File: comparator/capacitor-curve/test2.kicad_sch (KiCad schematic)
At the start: 4 parts

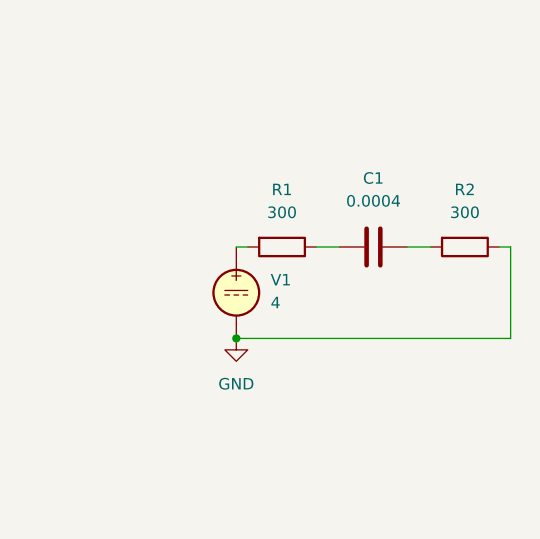
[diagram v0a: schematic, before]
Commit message: add/fix
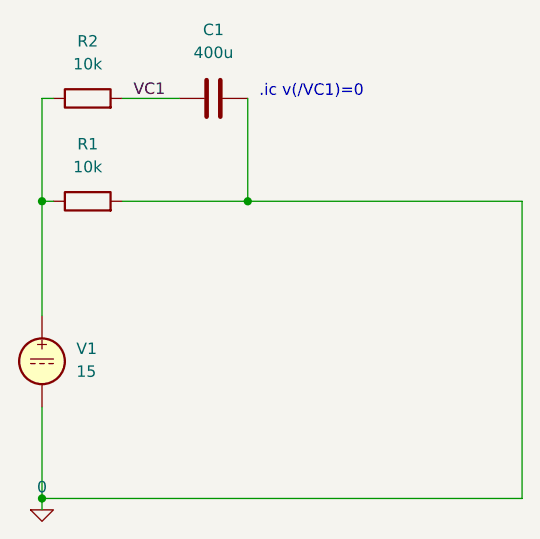
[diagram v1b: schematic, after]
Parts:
- C1: value 0.0004 -> 400u
- R1, R2: value 300 -> 10k
- V1: value 4 -> 15
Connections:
- net at R1.1: now also R2.1, V1.1; no longer C1.1
- net 0: now reaches C1.2
- net 0: now also R1.2, V1.2; no longer R2.2
- removed net GND: R2.1, V1.2
- new net VC1: C1.1, R2.2
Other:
- note added: ".ic v(/VC1)=0"
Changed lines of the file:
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@@
 (kicad_sch (version 20230121) (generator eeschema)
   (paper "A4")
-  (junction (at 81.28 90.17) (diameter 0) (color 0 0 0 0)
+  (junction (at 59.69 74.93) (diameter 0) (color 0 0 0 0)
   )
-  (wire (pts (xy 81.28 80.01) (xy 82.55 80.01))
+  (junction (at 82.55 74.93) (diameter 0) (color 0 0 0 0)
+  )
+  (junction (at 59.69 107.95) (diameter 0) (color 0 0 0 0)
+  )
+  (wire (pts (xy 113.03 107.95) (xy 113.03 74.93))
     (stroke (width 0) (type default))
   )
-  (wire (pts (xy 92.71 80.01) (xy 90.17 80.01))
+  (wire (pts (xy 59.69 109.22) (xy 59.69 107.95))
     (stroke (width 0) (type default))
   )
-  (wire (pts (xy 111.76 80.01) (xy 111.76 90.17))
+  (wire (pts (xy 59.69 87.63) (xy 59.69 74.93))
     (stroke (width 0) (type default))
   )
-  (wire (pts (xy 110.49 80.01) (xy 111.76 80.01))
+  (wire (pts (xy 59.69 97.79) (xy 59.69 107.95))
     (stroke (width 0) (type default))
   )
-  (wire (pts (xy 100.33 80.01) (xy 102.87 80.01))
+  (wire (pts (xy 59.69 74.93) (xy 60.96 74.93))
     (stroke (width 0) (type default))
   )
-  (wire (pts (xy 111.76 90.17) (xy 81.28 90.17))
+  (wire (pts (xy 59.69 63.5) (xy 60.96 63.5))
     (stroke (width 0) (type default))
   )
-  (symbol (lib_id "Device:C") (at 96.52 80.01 90) (unit 1)
+  (wire (pts (xy 82.55 74.93) (xy 113.03 74.93))
+    (stroke (width 0) (type default))
+  )
+  (wire (pts (xy 82.55 63.5) (xy 82.55 74.93))
+    (stroke (width 0) (type default))
+  )
+  (wire (pts (xy 59.69 74.93) (xy 59.69 63.5))
+    (stroke (width 0) (type default))
+  )
+  (wire (pts (xy 68.58 74.93) (xy 82.55 74.93))
+    (stroke (width 0) (type default))
+  )
+  (wire (pts (xy 59.69 107.95) (xy 113.03 107.95))
+    (stroke (width 0) (type default))
+  )
+  (wire (pts (xy 68.58 63.5) (xy 74.93 63.5))
+    (stroke (width 0) (type default))
+  )
+  (text ".ic v(/VC1)=0" (at 83.82 63.5 0)
+    (effects (font (size 1.27 1.27)) (justify left bottom))
+  )
+  (label "VC1" (at 69.85 63.5 0) (fields_autoplaced)
+    (effects (font (size 1.27 1.27)) (justify left bottom))
+  )
+  (symbol (lib_id "Simulation_SPICE:VDC") (at 59.69 92.71 0) (unit 1)
     (in_bom yes) (on_board yes) (dnp no) (fields_autoplaced)
-    (property "Reference" "C1" (at 96.52 72.39 90)
+    (property "Reference" "V1" (at 63.5 91.3102 0)
+      (effects (font (size 1.27 1.27)) (justify left))
+    )
+    (property "Value" "15" (at 63.5 93.8502 0)
+      (effects (font (size 1.27 1.27)) (justify left))
+    )
+    (property "Footprint" "" (at 59.69 92.71 0)
+      (effects (font (size 1.27 1.27)) hide)
+    )
+    (property "Datasheet" "~" (at 59.69 92.71 0)
+      (effects (font (size 1.27 1.27)) hide)
+    )
+    (property "Sim.Pins" "1=+ 2=-" (at 59.69 92.71 0)
+      (effects (font (size 1.27 1.27)) hide)
+    )
+    (property "Sim.Type" "DC" (at 59.69 92.71 0)
+      (effects (font (size 1.27 1.27)) hide)
+    )
+    (property "Sim.Device" "V" (at 59.69 92.71 0)
+      (effects (font (size 1.27 1.27)) (justify left) hide)
+    )
+    (pin "1")
+    (pin "2")
+    (instances
+      (project "test2"
+        (path "/bb173b4d-9621-4ad4-b8d6-5552f010e489"
+          (reference "V1") (unit 1)
+        )
+      )
+    )
+  )
+  (symbol (lib_id "Device:C") (at 78.74 63.5 90) (unit 1)
+    (in_bom yes) (on_board yes) (dnp no) (fields_autoplaced)
+    (property "Reference" "C1" (at 78.74 55.88 90)
       (effects (font (size 1.27 1.27)))
     )
-    (property "Value" "0.0004" (at 96.52 74.93 90)
+    (property "Value" "400u" (at 78.74 58.42 90)
       (effects (font (size 1.27 1.27)))
     )
-    (property "Footprint" "" (at 100.33 79.0448 0)
+    (property "Footprint" "" (at 82.55 62.5348 0)
       (effects (font (size 1.27 1.27)) hide)
     )
-    (property "Datasheet" "~" (at 96.52 80.01 0)
+    (property "Datasheet" "~" (at 78.74 63.5 0)
       (effects (font (size 1.27 1.27)) hide)
     )
@@
     (pin "2")
     (instances
-      (project "test-details"
-        (path "/8300bb89-af22-40bb-96f5-ff500b49d277"
+      (project "test2"
+        (path "/bb173b4d-9621-4ad4-b8d6-5552f010e489"
           (reference "C1") (unit 1)
         )
@@
     )
   )
-  (symbol (lib_id "Device:R") (at 106.68 80.01 270) (unit 1)
+  (symbol (lib_id "Device:R") (at 64.77 63.5 90) (unit 1)
     (in_bom yes) (on_board yes) (dnp no) (fields_autoplaced)
-    (property "Reference" "R2" (at 106.68 73.66 90)
+    (property "Reference" "R2" (at 64.77 57.15 90)
       (effects (font (size 1.27 1.27)))
     )
-    (property "Value" "300" (at 106.68 76.2 90)
+    (property "Value" "10k" (at 64.77 59.69 90)
       (effects (font (size 1.27 1.27)))
     )
-    (property "Footprint" "" (at 106.68 78.232 90)
+    (property "Footprint" "" (at 64.77 65.278 90)
       (effects (font (size 1.27 1.27)) hide)
     )
-    (property "Datasheet" "~" (at 106.68 80.01 0)
+    (property "Datasheet" "~" (at 64.77 63.5 0)
       (effects (font (size 1.27 1.27)) hide)
     )
@@
     (pin "2")
     (instances
-      (project "test-details"
-        (path "/8300bb89-af22-40bb-96f5-ff500b49d277"
+      (project "test2"
+        (path "/bb173b4d-9621-4ad4-b8d6-5552f010e489"
           (reference "R2") (unit 1)
         )
@@
     )
   )
-  (symbol (lib_id "Simulation_SPICE:VDC") (at 81.28 85.09 0) (unit 1)
+  (symbol (lib_id "Simulation_SPICE:0") (at 59.69 109.22 0) (unit 1)
     (in_bom yes) (on_board yes) (dnp no) (fields_autoplaced)
-    (property "Reference" "V1" (at 85.09 83.6902 0)
-      (effects (font (size 1.27 1.27)) (justify left))
-    )
-    (property "Value" "4" (at 85.09 86.2302 0)
-      (effects (font (size 1.27 1.27)) (justify left))
-    )
-    (property "Footprint" "" (at 81.28 85.09 0)
+    (property "Reference" "#GND01" (at 59.69 111.76 0)
       (effects (font (size 1.27 1.27)) hide)
     )
-    (property "Datasheet" "~" (at 81.28 85.09 0)
+    (property "Value" "0" (at 59.69 106.68 0)
+      (effects (font (size 1.27 1.27)))
+    )
+    (property "Footprint" "" (at 59.69 109.22 0)
       (effects (font (size 1.27 1.27)) hide)
     )
-    (property "Sim.Pins" "1=+ 2=-" (at 81.28 85.09 0)
+    (property "Datasheet" "~" (at 59.69 109.22 0)
       (effects (font (size 1.27 1.27)) hide)
     )
-    (property "Sim.Type" "DC" (at 81.28 85.09 0)
-      (effects (font (size 1.27 1.27)) hide)
-    )
-    (property "Sim.Device" "V" (at 81.28 85.09 0)
-      (effects (font (size 1.27 1.27)) (justify left) hide)
-    )
     (pin "1")
-    (pin "2")
     (instances
-      (project "test-details"
-        (path "/8300bb89-af22-40bb-96f5-ff500b49d277"
-          (reference "V1") (unit 1)
+      (project "test2"
+        (path "/bb173b4d-9621-4ad4-b8d6-5552f010e489"
+          (reference "#GND01") (unit 1)
         )
       )
     )
   )
-  (symbol (lib_id "Device:R") (at 86.36 80.01 270) (unit 1)
+  (symbol (lib_id "Device:R") (at 64.77 74.93 90) (unit 1)
     (in_bom yes) (on_board yes) (dnp no) (fields_autoplaced)
-    (property "Reference" "R1" (at 86.36 73.66 90)
+    (property "Reference" "R1" (at 64.77 68.58 90)
       (effects (font (size 1.27 1.27)))
     )
-    (property "Value" "300" (at 86.36 76.2 90)
+    (property "Value" "10k" (at 64.77 71.12 90)
       (effects (font (size 1.27 1.27)))
     )
-    (property "Footprint" "" (at 86.36 78.232 90)
+    (property "Footprint" "" (at 64.77 76.708 90)
       (effects (font (size 1.27 1.27)) hide)
     )
-    (property "Datasheet" "~" (at 86.36 80.01 0)
+    (property "Datasheet" "~" (at 64.77 74.93 0)
       (effects (font (size 1.27 1.27)) hide)
     )
@@
     (pin "2")
     (instances
-      (project "test-details"
-        (path "/8300bb89-af22-40bb-96f5-ff500b49d277"
+      (project "test2"
+        (path "/bb173b4d-9621-4ad4-b8d6-5552f010e489"
           (reference "R1") (unit 1)
         )
       )
-    )
-  )
-  (symbol (lib_id "power:GND") (at 81.28 90.17 0) (unit 1)
-    (in_bom yes) (on_board yes) (dnp no) (fields_autoplaced)
-    (property "Reference" "#PWR01" (at 81.28 96.52 0)
-      (effects (font (size 1.27 1.27)) hide)
-    )
-    (property "Value" "GND" (at 81.28 95.25 0)
-      (effects (font (size 1.27 1.27)))
-    )
-    (property "Footprint" "" (at 81.28 90.17 0)
-      (effects (font (size 1.27 1.27)) hide)
-    )
-    (property "Datasheet" "" (at 81.28 90.17 0)
-      (effects (font (size 1.27 1.27)) hide)
-    )
-    (pin "1")
-    (instances
-      (project "test-details"
-        (path "/8300bb89-af22-40bb-96f5-ff500b49d277"
-          (reference "#PWR01") (unit 1)
-        )
-      )
